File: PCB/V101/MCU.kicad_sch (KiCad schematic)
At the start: 26 parts, among them SW501 SW_Push, SW502 SW_Push, SW503 SW_Push, U501 STM32G431CBUx, Y501 Crystal_GND24, Y502 Crystal_GND24

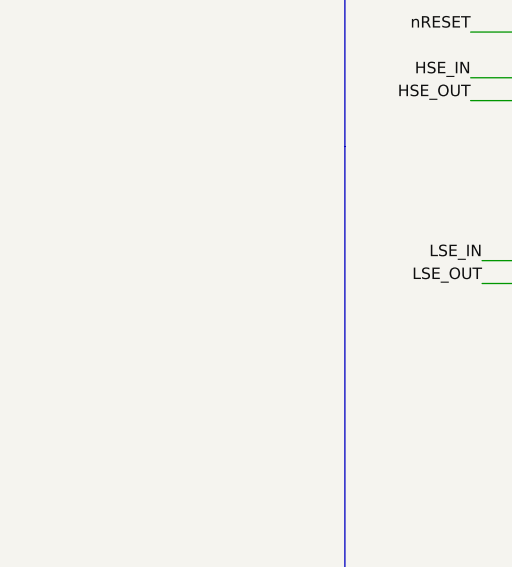
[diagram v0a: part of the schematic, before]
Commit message: Updated PCB
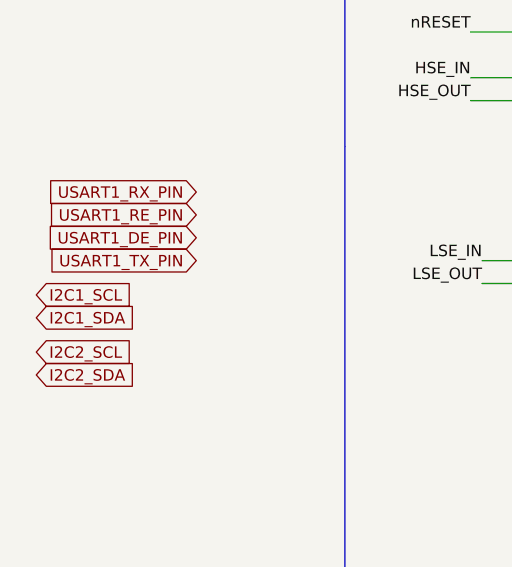
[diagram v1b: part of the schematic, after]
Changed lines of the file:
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@@
+		)
+	)
+	(global_label "I2C1_SCL"
+		(shape input)
+		(at -20.32 77.47 0)
+		(fields_autoplaced yes)
+		(effects
+			(font
+				(size 1.27 1.27)
+			)
+			(justify left)
+		)
+		(property "Intersheetrefs" "${INTERSHEET_REFS}"
+			(at -8.5658 77.47 0)
+			(effects
+				(font
+					(size 1.27 1.27)
+				)
+				(justify left)
+				(hide yes)
+			)
+		)
+	)
+	(global_label "I2C1_SDA"
+		(shape input)
+		(at -20.32 80.01 0)
+		(fields_autoplaced yes)
+		(effects
+			(font
+				(size 1.27 1.27)
+			)
+			(justify left)
+		)
+		(property "Intersheetrefs" "${INTERSHEET_REFS}"
+			(at -8.5053 80.01 0)
+			(effects
+				(font
+					(size 1.27 1.27)
+				)
+				(justify left)
+				(hide yes)
+			)
+		)
+	)
+	(global_label "I2C2_SDA"
+		(shape input)
+		(at -20.32 86.36 0)
+		(fields_autoplaced yes)
+		(effects
+			(font
+				(size 1.27 1.27)
+			)
+			(justify left)
+		)
+		(property "Intersheetrefs" "${INTERSHEET_REFS}"
+			(at -8.5053 86.36 0)
+			(effects
+				(font
+					(size 1.27 1.27)
+				)
+				(justify left)
+				(hide yes)
+			)
+		)
+	)
+	(global_label "USART1_DE_PIN"
+		(shape input)
+		(at -2.54 71.12 180)
+		(fields_autoplaced yes)
+		(effects
+			(font
+				(size 1.27 1.27)
+			)
+			(justify right)
+		)
+		(property "Intersheetrefs" "${INTERSHEET_REFS}"
+			(at -20.1604 71.12 0)
+			(effects
+				(font
+					(size 1.27 1.27)
+				)
+				(justify right)
+				(hide yes)
+			)
+		)
+	)
+	(global_label "USART1_RE_PIN"
+		(shape input)
+		(at -2.54 68.58 180)
+		(fields_autoplaced yes)
+		(effects
+			(font
+				(size 1.27 1.27)
+			)
+			(justify right)
+		)
+		(property "Intersheetrefs" "${INTERSHEET_REFS}"
+			(at -20.1604 68.58 0)
+			(effects
+				(font
+					(size 1.27 1.27)
+				)
+				(justify right)
+				(hide yes)
+			)
+		)
+	)
+	(global_label "I2C2_SCL"
+		(shape input)
+		(at -20.32 83.82 0)
+		(fields_autoplaced yes)
+		(effects
+			(font
+				(size 1.27 1.27)
+			)
+			(justify left)
+		)
+		(property "Intersheetrefs" "${INTERSHEET_REFS}"
+			(at -8.5658 83.82 0)
+			(effects
+				(font
+					(size 1.27 1.27)
+				)
+				(justify left)
+				(hide yes)
+			)
+		)
+	)
+	(global_label "USART1_TX_PIN"
+		(shape input)
+		(at -2.54 73.66 180)
+		(fields_autoplaced yes)
+		(effects
+			(font
+				(size 1.27 1.27)
+			)
+			(justify right)
+		)
+		(property "Intersheetrefs" "${INTERSHEET_REFS}"
+			(at -19.9185 73.66 0)
+			(effects
+				(font
+					(size 1.27 1.27)
+				)
+				(justify right)
+				(hide yes)
+			)
+		)
+	)
+	(global_label "USART1_RX_PIN"
+		(shape input)
+		(at -2.54 66.04 180)
+		(fields_autoplaced yes)
+		(effects
+			(font
+				(size 1.27 1.27)
+			)
+			(justify right)
+		)
+		(property "Intersheetrefs" "${INTERSHEET_REFS}"
+			(at -20.2209 66.04 0)
+			(effects
+				(font
+					(size 1.27 1.27)
+				)
+				(justify right)
+				(hide yes)
+			)
 		)
 	)
